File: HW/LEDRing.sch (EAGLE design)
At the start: 43 parts, among them U1 ATMEGA328P-AU, U2 MCP73831, U3 MIC5219 3.3V, U4 MMA8452Q, Y1 16MHZ

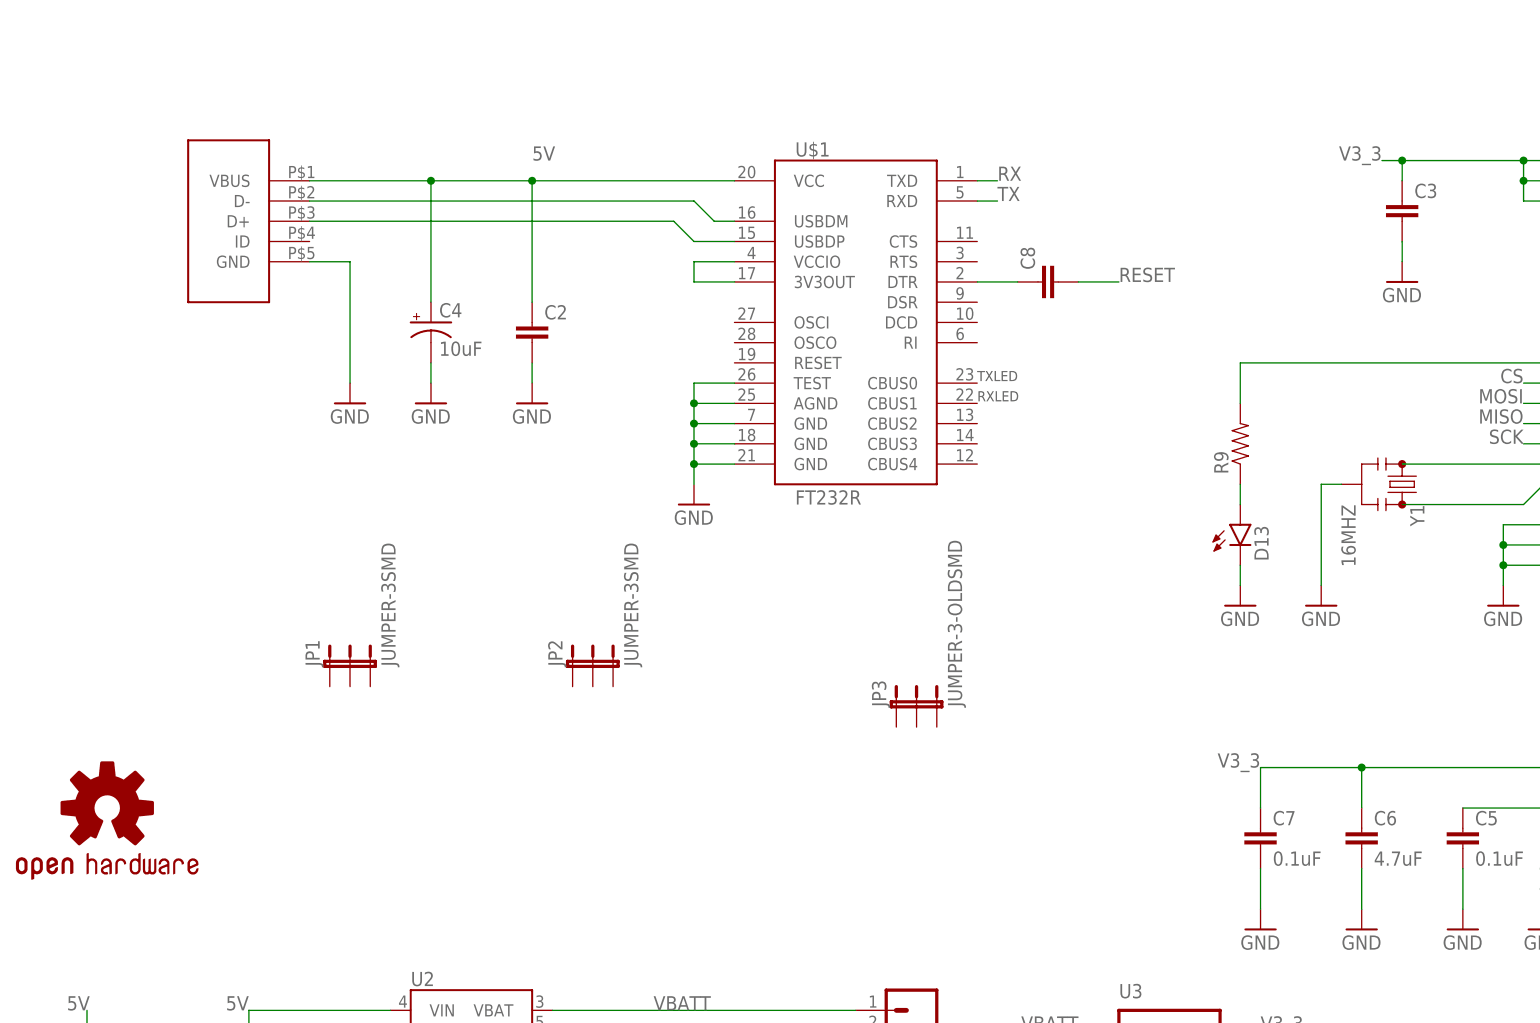
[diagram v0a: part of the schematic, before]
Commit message: Updated to version 1.1.
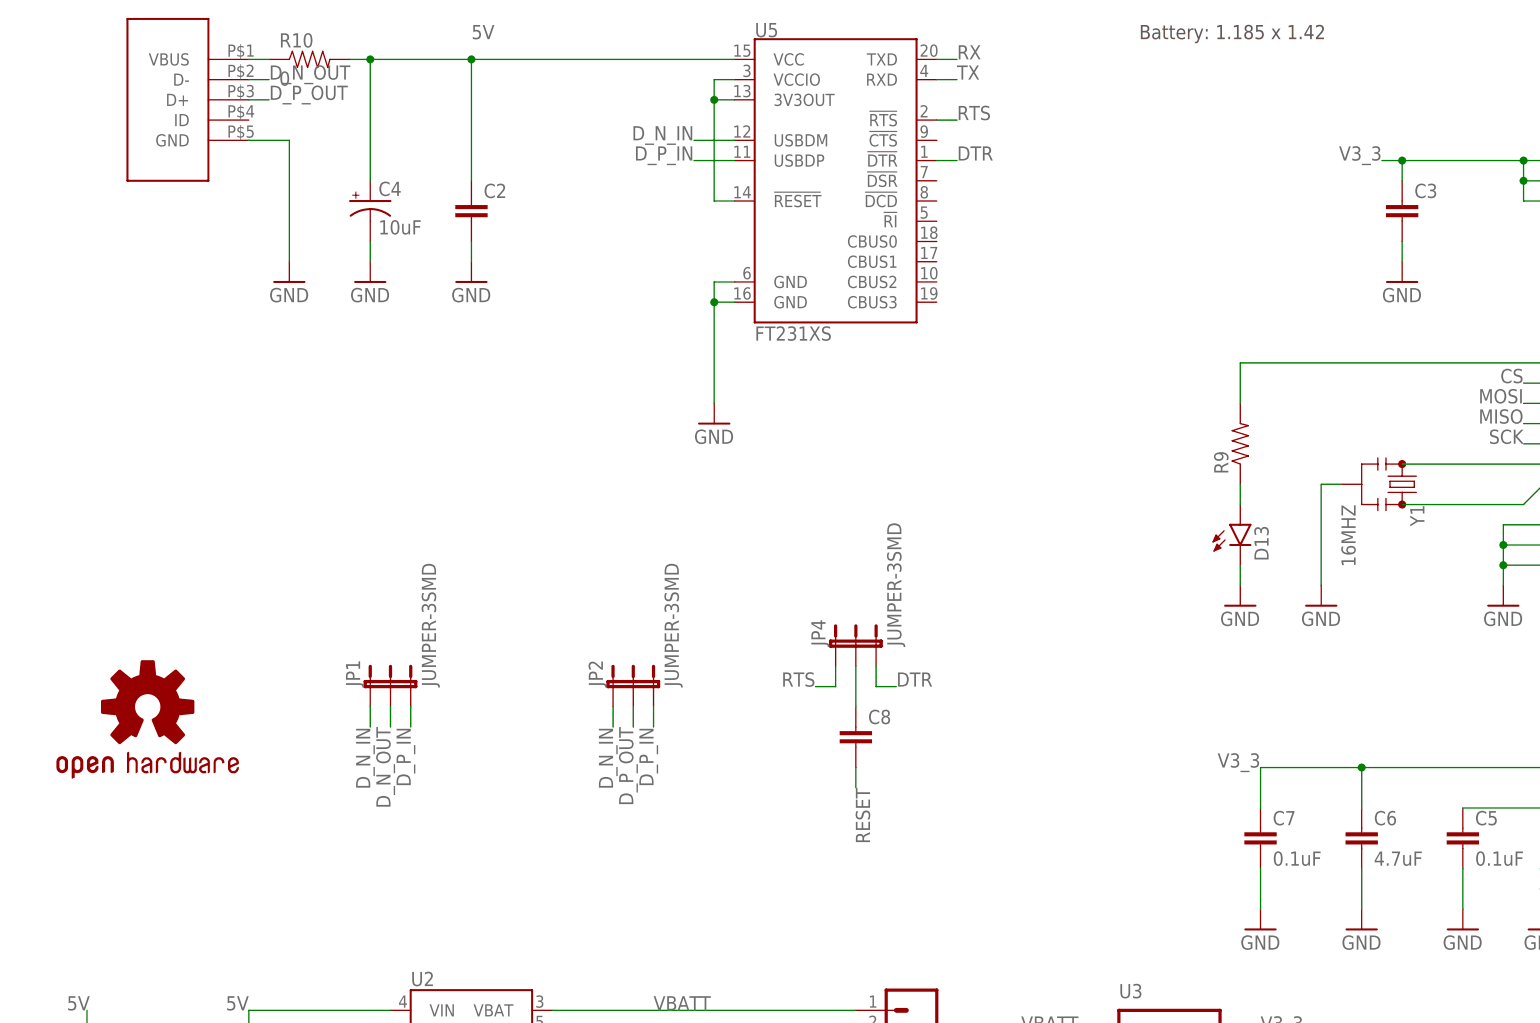
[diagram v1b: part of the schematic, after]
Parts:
- removed JP3: JUMPER-3-OLDSMD, SparkFun-Retired:JUMPER-3-OLDSMD
- removed U$1: FT232R, GeekAmmo:FT232R
- added JP4: JUMPER-3SMD, SparkFun-Retired:JUMPER-3SMD
- added R10: 0, SparkFun-Passives:RESISTOR0603-RES
- added U5: FT231XS, SparkFun-DigitalIC:FT231XS
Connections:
- removed net N$31: U$1.3V3OUT, U$1.VCCIO
- removed net N$32: C8.1, U$1.DTR
- new net DTR: JP4.3, U5.!DTR
- new net D_N_IN: JP1.1, JP2.1, U5.USBDM
- new net D_N_OUT: JP1.2, U$2.D-
- new net D_P_IN: JP1.3, JP2.3, U5.USBDP
- new net D_P_OUT: JP2.2, U$2.D+
- new net RTS: JP4.1, U5.!RTS
- new net RTS_OR_DTR: C8.1, JP4.2
- net 5V: now also R10.2, U5.VCC; no longer U$1.VCC, U$2.VBUS
- net GND: now also U5.GND@16, U5.GND@6; no longer U$1.AGND, U$1.GND@18, U$1.GND@21, U$1.GND@7, U$1.TEST
- net N$4: now also R10.1, U$2.VBUS; no longer U$1.USBDM, U$2.D-
- net N$5: now also U5.!RESET, U5.3V3OUT, U5.VCCIO; no longer U$1.USBDP, U$2.D+
- net RX: now also U5.TXD; no longer U$1.TXD
- net TX: now also U5.RXD; no longer U$1.RXD
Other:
- note added: "Battery: 1.185 x 1.42"
- moved on the sheet: C2, C4, C8, JP1, JP2
